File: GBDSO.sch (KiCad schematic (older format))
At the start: 0 parts

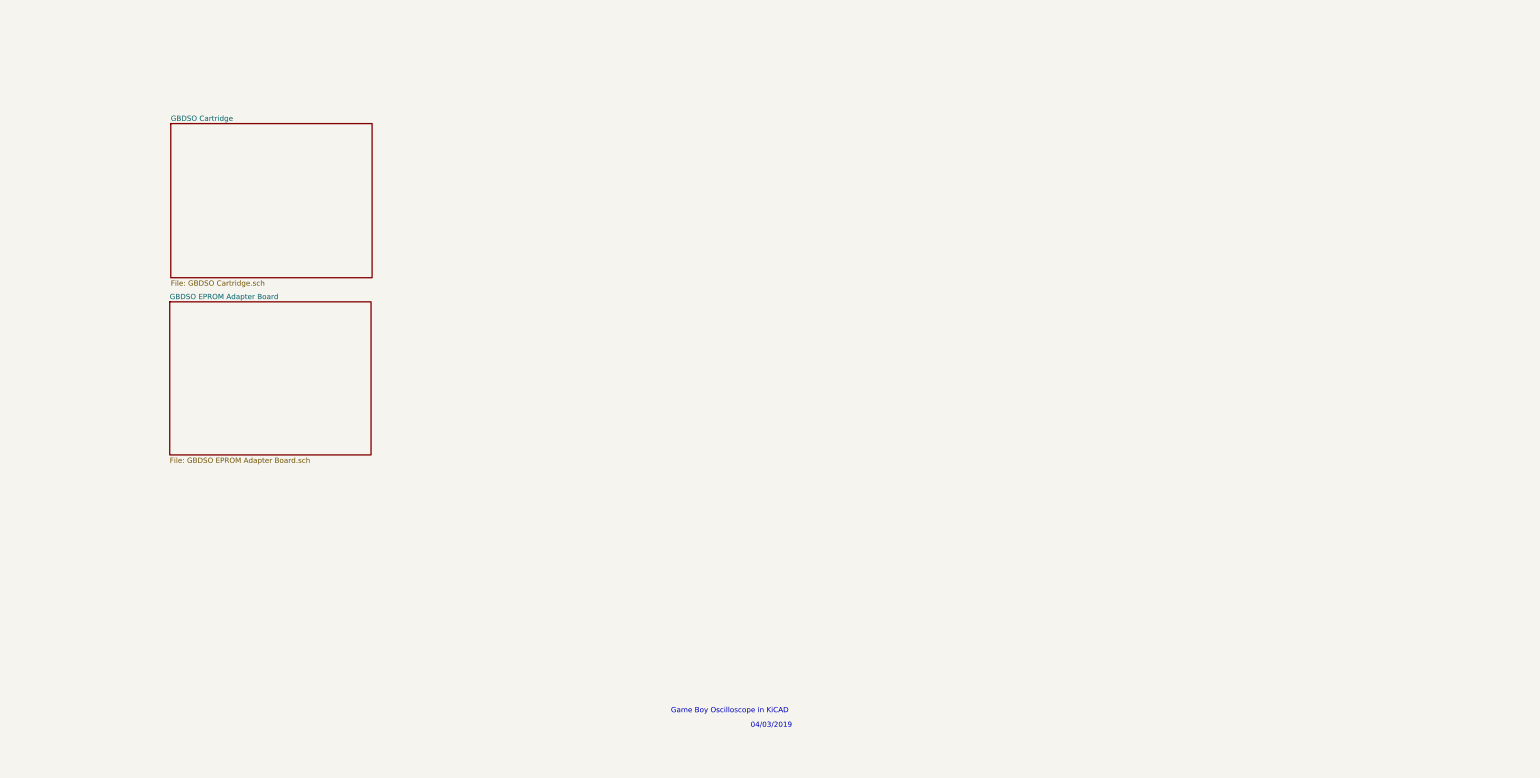
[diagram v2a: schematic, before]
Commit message: big v2 update, hopefully everything is ok now
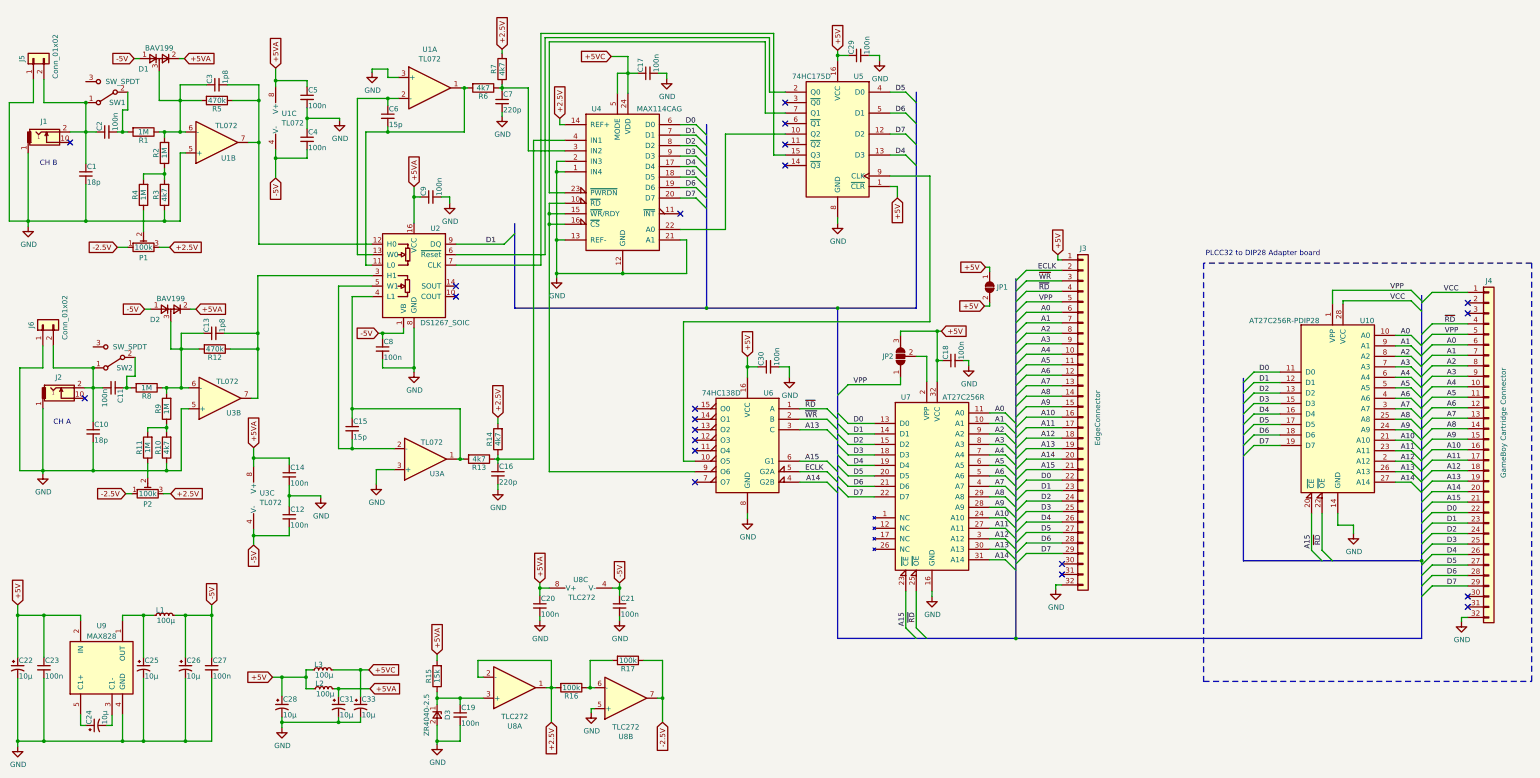
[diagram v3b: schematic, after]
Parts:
- added C1, C10: 18p, Capacitor_SMD:C_0805_2012Metric, symbol Device:C_Small
- added C11, C12, C14, C17, C18, C19, C2, C20, C21, C23, C27, C29, C30, C4, C5, C8, C9: 100n, Capacitor_SMD:C_0805_2012Metric, symbol Device:C_Small
- added C13, C3: 1p8, Capacitor_SMD:C_0805_2012Metric, symbol Device:C_Small
- added C15, C6: 15p, Capacitor_SMD:C_0805_2012Metric, symbol Device:C_Small
- added C16, C7: 220p, Capacitor_SMD:C_0805_2012Metric, symbol Device:C_Small
- added C22, C24, C25, C26, C28, C31, C33: 10µ, Capacitor_SMD:C_1206_3216Metric, symbol Device:C_Polarized_Small_US
- added D1, D2: BAV199, Package_TO_SOT_SMD:SOT-23_Handsoldering, symbol BAV199:BAV199
- added D3: ZR4040-2.5, Package_TO_SOT_SMD:SOT-23_Handsoldering, symbol ZR40402F25TA:ZR4040-2.5
- added J1, J2: MJ-3523-SMT-TR, MJ-3523-SMT-TR:MJ-3523-SMT-TR, symbol MJ-3523-SMT-TR:MJ-3523-SMT-TR
- added J3: EdgeConnector, GB_EdgeConnector:GB_EdgeConnector, symbol Connector_Generic:Conn_01x32
- added J4: GameBoy Cartridge Connector, Game_Boy_Cartridge_Slot_Xunbeifang_GNI172:Game_Boy_Cartridge_Slot_Xunbeifang_GNI172, symbol Connector_Generic:Conn_01x32
- added J5, J6: Conn_01x02, Connector_PinHeader_2.54mm:PinHeader_1x02_P2.54mm_Horizontal, symbol Connector_Generic:Conn_01x02
- added JP1: SolderJumper_2_Open, Jumper:SolderJumper-2_P1.3mm_Open_TrianglePad1.0x1.5mm, symbol Jumper:SolderJumper_2_Open
- added JP2: SolderJumper_3_Open, Jumper:SolderJumper-3_P1.3mm_Open_RoundedPad1.0x1.5mm_NumberLabels, symbol Jumper:SolderJumper_3_Open
- added L1, L2, L3: 100µ, Inductor_SMD:L_0805_2012Metric_Pad1.15x1.40mm_HandSolder, symbol Device:L_Small
- added P1, P2: 100k, Potentiometer_SMD:Potentiometer_Vishay_TS53YJ_Vertical, symbol Device:R_Potentiometer_Trim
- added R1, R11, R2, R4, R8, R9: 1M, Resistor_SMD:R_0805_2012Metric, symbol Device:R
- added R10, R13, R14, R3, R6, R7: 4k7, Resistor_SMD:R_0805_2012Metric, symbol Device:R
- added R12, R5: 470k, Resistor_SMD:R_0805_2012Metric, symbol Device:R
- added R15: 15k, Resistor_SMD:R_0805_2012Metric, symbol Device:R
- added R16, R17: 100k, Resistor_SMD:R_0805_2012Metric, symbol Device:R
- added SW1, SW2: SW_SPDT, Button_Switch_SMD:SW_SPDT_CK-JS102011SAQN, symbol Switch:SW_SPDT
- added U1, U3: TL072, Package_SO:SOIC-8_3.9x4.9mm_P1.27mm, symbol Amplifier_Operational:TL072
- added U10: AT27C256R-PDIP28, Package_DIP:DIP-28_W15.24mm_Socket_LongPads, symbol AT27C256R:AT27C256R-PDIP28
- added U2: DS1267_SOIC, Package_SO:SOIC-16W_7.5x10.3mm_P1.27mm, symbol Potentiometer_Digital:DS1267_SOIC
- added U4: MAX114CAG, Package_SO:SSOP-24_5.3x8.2mm_P0.65mm, symbol MAX114CAG:MAX114CAG
- added U5: 74HC175D, Package_SO:SOIC-16_3.9x9.9mm_P1.27mm, symbol 74HC175D:74HC175D
- added U6: 74HC138D, Package_SO:SOIC-16_3.9x9.9mm_P1.27mm, symbol 74HC138D:74HC138D
- added U7: AT27C256R, PLCC32_HandSolder:PLCC-32_HandSolder, symbol AT27C256R:AT27C256R
- added U8: TLC272, Package_SO:SOIC-8_3.9x4.9mm_P1.27mm, symbol Amplifier_Operational:TLC272
- added U9: MAX828, Package_TO_SOT_SMD:SOT-23-5_HandSoldering, symbol MAX828EUK:MAX828
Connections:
- new net: C6.2, R6.2, U1.1, U2.11 (L0)
- new net: C3.2, R5.1, U1.7, U2.12 (H0)
- new net: C6.1, U1.2 (-), U2.13 (W0)
- new net: C13.2, R12.1, U2.3 (H1), U3.7
- new net: C15.1, R13.2, U2.4 (L1), U3.1
- new net: C15.2, U2.5 (W1), U3.2 (-)
- new net: U2.6 (~Reset), U5.2 (Q0)
- new net: U2.7 (CLK), U5.15 (Q3)
- new net: C3.1, D1.3, R1.1, R2.2, R5.2, U1.6 (-)
- new net: C2.2, R1.2, SW1.2 (B)
- new net: R2.1, R3.2, R4.2
- new net: C13.1, D2.3, R12.2, R8.1, R9.2, U3.6 (-)
- new net: C11.1, R8.2, SW2.2 (B)
- new net: R10.2, R11.2, R9.1
- new net: P2.2, R11.1
- new net: C19.1, D3.1, R15.1, U8.3 (+)
- new net: C7.1, R6.1, R7.1, U4.3 (IN2)
- new net: C16.1, R13.1, R14.1, U4.4 (IN1)
- new net: R16.1, R17.2, U8.6 (-)
- new net: C1.1, C2.1, J1.2, J5.2 (Pin_2), SW1.1 (A)
- new net: C10.1, C11.2, J2.2, J6.2 (Pin_2), SW2.1 (A)
- new net: C24.1, U9.5 (C1+)
- new net: C24.2, U9.3 (C1-)
- new net: C25.1, L1.1, U9.1 (OUT)
- new net: P1.2, R4.1
- new net: U4.10 (~RD), U4.15 (~WR~/RDY), U4.16 (~CS), U6.9 (O6)
- new net: U4.22 (A0), U5.10 (Q2)
- new net: U4.23 (~PWRDN), U5.7 (Q1)
- new net: U5.9 (CLK), U6.10 (O5)
- new net: JP2.2 (C), U7.2 (VPP)
- new net +2.5V: P1.3, P2.3, R14.2, R16.2, R7.2, U4.14 (REF+), U8.1, U8.2 (-)
- new net +5V: C18.1, C22.1, C23.1, C28.1, C29.1, C30.1, J3.1 (Pin_1), JP1.1 (A), JP1.2 (B), JP2.3 (B), L2.1, L3.1, U5.1 (~CLR), U5.16 (VCC), U6.16 (VCC), U7.32 (VCC), U9.2 (IN)
- new net +5VA: C14.1, C20.1, C31.1, C5.1, C9.1, D1.2, D2.2, L2.2, R15.2, U1.8 (V+), U2.16 (VCC), U3.8 (V+), U8.8 (V+)
- new net +5VC: C17.1, C33.1, L3.2, U4.24 (VDD), U4.5 (MODE)
- new net -2.5V: P1.1, P2.1, R17.1, U8.7
- new net -5V: C12.2, C21.1, C26.1, C27.1, C4.2, C8.1, D1.1, D2.1, L1.2, U1.4 (V-), U2.1 (VB), U3.4 (V-), U8.4 (V-)
- new net A0: J3.6 (Pin_6), J4.6 (Pin_6), U10.10 (A0), U7.11 (A0)
- new net A1: J3.7 (Pin_7), J4.7 (Pin_7), U10.9 (A1), U7.10 (A1)
- new net A10: J3.16 (Pin_16), J4.16 (Pin_16), U10.21 (A10), U7.24 (A10)
- new net A11: J3.17 (Pin_17), J4.17 (Pin_17), U10.23 (A11), U7.27 (A11)
- new net A12: J3.18 (Pin_18), J4.18 (Pin_18), U10.2 (A12), U7.3 (A12)
- new net A13: J3.19 (Pin_19), J4.19 (Pin_19), U10.26 (A13), U6.3 (C), U7.30 (A13)
- new net A14: J3.20 (Pin_20), J4.20 (Pin_20), U10.27 (A14), U6.4 (G2B), U7.31 (A14)
- new net A15: J3.21 (Pin_21), J4.21 (Pin_21), U10.20 (~CE), U6.6 (G1), U7.23 (~CE)
- new net A2: J3.8 (Pin_8), J4.8 (Pin_8), U10.8 (A2), U7.9 (A2)
- new net A3: J3.9 (Pin_9), J4.9 (Pin_9), U10.7 (A3), U7.8 (A3)
- new net A4: J3.10 (Pin_10), J4.10 (Pin_10), U10.6 (A4), U7.7 (A4)
- new net A5: J3.11 (Pin_11), J4.11 (Pin_11), U10.5 (A5), U7.6 (A5)
- new net A6: J3.12 (Pin_12), J4.12 (Pin_12), U10.4 (A6), U7.5 (A6)
- new net A7: J3.13 (Pin_13), J4.13 (Pin_13), U10.3 (A7), U7.4 (A7)
- new net A8: J3.14 (Pin_14), J4.14 (Pin_14), U10.25 (A8), U7.29 (A8)
- new net A9: J3.15 (Pin_15), J4.15 (Pin_15), U10.24 (A9), U7.28 (A9)
- new net D0: J3.22 (Pin_22), J4.22 (Pin_22), U10.11 (D0), U4.6 (D0), U7.13 (D0)
- new net D1: J3.23 (Pin_23), J4.23 (Pin_23), U10.12 (D1), U2.9 (DQ), U4.7 (D1), U7.14 (D1)
- new net D2: J3.24 (Pin_24), J4.24 (Pin_24), U10.13 (D2), U4.8 (D2), U7.15 (D2)
- new net D3: J3.25 (Pin_25), J4.25 (Pin_25), U10.15 (D3), U4.9 (D3), U7.18 (D3)
- new net D4: J3.26 (Pin_26), J4.26 (Pin_26), U10.16 (D4), U4.17 (D4), U5.13 (D3), U7.19 (D4)
- new net D5: J3.27 (Pin_27), J4.27 (Pin_27), U10.17 (D5), U4.18 (D5), U5.4 (D0), U7.20 (D5)
- new net D6: J3.28 (Pin_28), J4.28 (Pin_28), U10.18 (D6), U4.19 (D6), U5.5 (D1), U7.21 (D6)
- new net D7: J3.29 (Pin_29), J4.29 (Pin_29), U10.19 (D7), U4.20 (D7), U5.12 (D2), U7.22 (D7)
- new net ECLK: J3.2 (Pin_2), U6.5 (G2A)
- new net GND: C1.2, C10.2, C12.1, C14.2, C16.2, C17.2, C18.2, C19.2, C20.2, C21.2, C22.2, C23.2, C25.2, C26.2, C27.2, C28.2, C29.2, C30.2, C31.2, C33.2, C4.1, C5.2, C7.2, C8.2, C9.2, D3.2, J1.1, J2.1, J3.32 (Pin_32), J4.32 (Pin_32), J5.1 (Pin_1), J6.1 (Pin_1), R10.1, R3.1, U1.3 (+), U1.5 (+), U10.14 (GND), U2.8 (GND), U3.3 (+), U3.5 (+), U4.1 (IN4), U4.12 (GND), U4.13 (REF-), U4.2 (IN3), U4.21 (A1), U5.8 (GND), U6.8 (GND), U7.16 (GND), U8.5 (+), U9.4 (GND)
- new net VCC: J4.1 (Pin_1), U10.28 (VCC)
- new net VPP: J3.5 (Pin_5), J4.5 (Pin_5), JP2.1 (A), U10.1 (VPP)
- new net ~RD: J3.4 (Pin_4), J4.4 (Pin_4), U10.22 (~OE), U6.1 (A), U7.25 (~OE)
- new net ~WR: J3.3 (Pin_3), U6.2 (B)
- no-connect marks 0 -> 21
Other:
- note added: "CH A"
- note added: "CH B"
- note added: "PLCC32 to DIP28 Adapter board"
- note removed: "04/03/2019"
- note removed: "Game Boy Oscilloscope in KiCAD"
